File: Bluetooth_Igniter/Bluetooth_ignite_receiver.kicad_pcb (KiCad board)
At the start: 2 copper layers, 69 parts, among them J1 Screw_Terminal_01x02, J2 Screw_Terminal_01x02, J3 Screw_Terminal_01x02, J4 Screw_Terminal_01x02, J5 USB_C_Receptacle_USB2.0, Q1 MMDT2222A, Q2 MMDT2222A, Q3 Q_NMOS_GSD, Q4 Q_NMOS_GSD, SW1 SW_Push, SW2 SW_Push, U1 CP2102N-A01-GQFN24, U2 ESP32-WROOM-32, U3 LTV-817S, U4 LTV-817S, U5 TPS63060

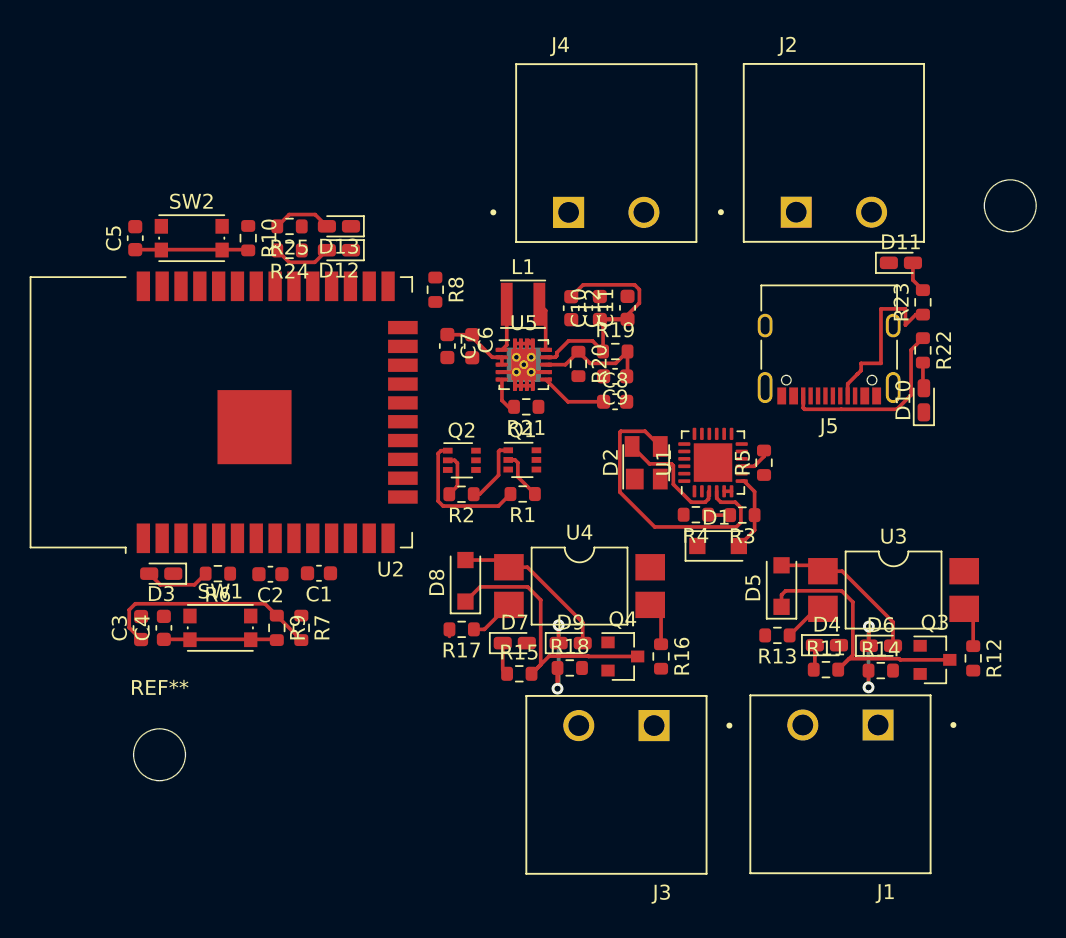
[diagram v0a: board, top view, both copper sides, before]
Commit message: pcb routing
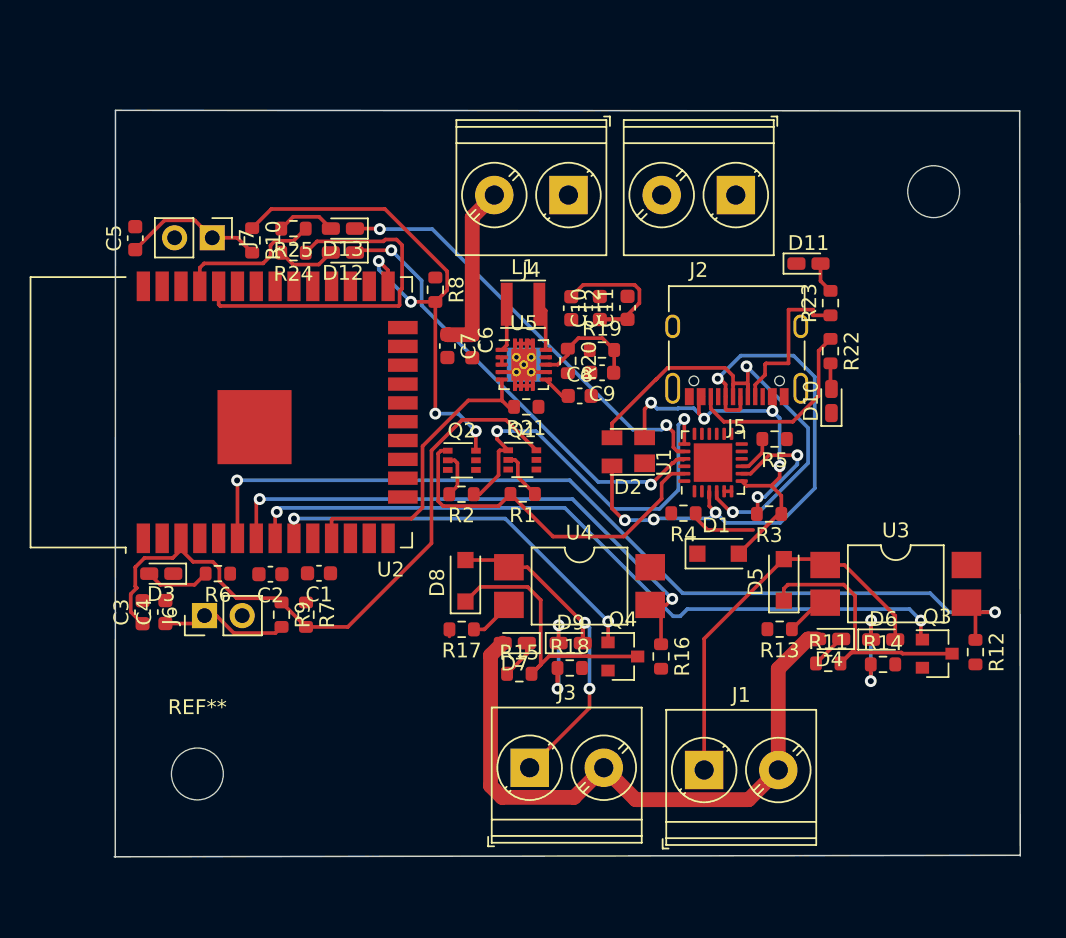
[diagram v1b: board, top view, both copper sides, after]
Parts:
- removed SW1, SW2: SW_Push, Button_Switch_SMD:SW_Push_1P1T_NO_CK_KMR2
- added J6: Conn_01x02_Male, Connector_PinHeader_2.54mm:PinHeader_1x02_P2.54mm_Vertical, F.Cu at (32.7, 115.3)
- added J7: Conn_01x02_Male, Connector_PinHeader_2.54mm:PinHeader_1x02_P2.54mm_Vertical, F.Cu at (33.2, 89.8)
- J1, J2, J3, J4: footprint iclrhw:PHOENIX_1757242 -> TerminalBlock_Phoenix:TerminalBlock_Phoenix_PT-1,5-2-5.0-H_1x02_P5.00mm_Horizontal
- moved J1 9.25 mm to (66.4, 125.7), turned to 0 degrees
- moved J2 7.20 mm to (68.5, 86.9), turned to 180 degrees
- moved D10 6.24 mm to (75.0, 100.8)
- moved D11 6.24 mm to (73.4, 91.6)
- moved J5 6.24 mm to (68.6, 96.9)
- moved R22 6.24 mm to (74.9, 97.5)
- moved R23 6.24 mm to (74.9, 94.2)
- moved J3 5.97 mm to (54.6, 125.6), turned to 0 degrees
- moved REF** 5.26 mm to (81.9, 86.7)
- moved J4 3.81 mm to (57.3, 86.9), turned to 180 degrees
- moved REF** 2.86 mm to (32.2, 126.0)
- moved C8 2.42 mm to (58.0, 100.5)
- moved R3 1.81 mm to (70.8, 108.5)
- moved R5 1.75 mm to (71.2, 103.4), turned to 180 degrees
- moved D2 1.41 mm to (61.3, 104.3), turned to 180 degrees
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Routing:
- net /Cont1: track 2.77 -> 63.7 mm, vias 0 -> 2
- net /Nuke1: track 0.00 -> 50.3 mm, vias 0 -> 2
- net /pyros/Ext_supply: track 0.00 -> 43.8 mm
- net /BOOT: track 0.00 -> 37.2 mm, vias 0 -> 4
- net /Cont2: track 2.96 -> 38.0 mm, vias 0 -> 2
- net /usb/D+: track 8.08 -> 39.9 mm, vias 0 -> 4
- net /TXD: track 0.00 -> 30.5 mm, vias 0 -> 2
- net /EN: track 15.1 -> 45.6 mm
- net /RXD: track 0.00 -> 29.3 mm, vias 0 -> 2
- net /Nuke2: track 0.00 -> 26.8 mm, vias 0 -> 2
- net Net-(R24-Pad1): track 0.00 -> 24.6 mm
- net /RTS: track 4.50 -> 27.7 mm, vias 0 -> 2
- net /usb/VBUS: track 5.27 -> 28.3 mm, vias 0 -> 4
- net /PG: track 2.46 -> 21.0 mm
- net Net-(D5-Pad2): track 10.7 -> 27.2 mm
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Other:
- board outline added: 61.1 x 50.4 mm
